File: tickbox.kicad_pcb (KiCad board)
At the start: 2 copper layers, 1 part, among them IC1 R5F10RLAGFB#10

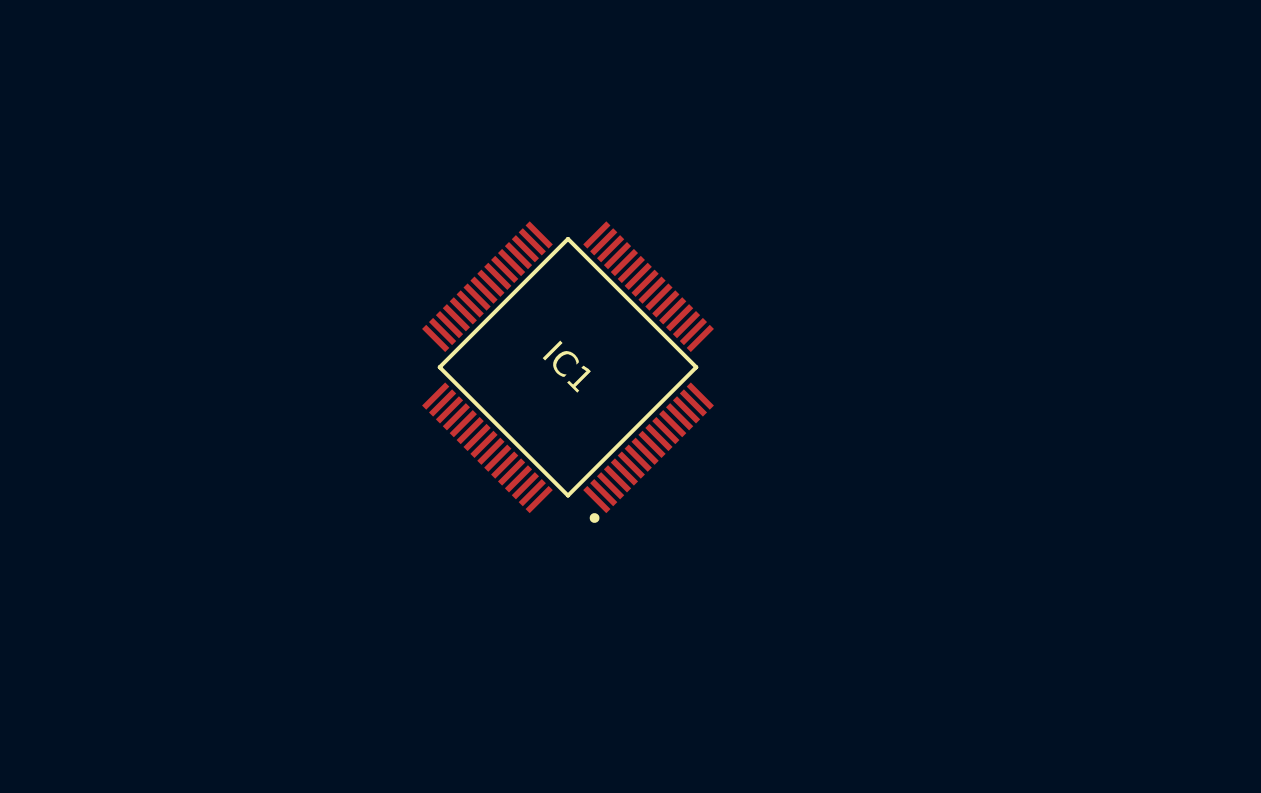
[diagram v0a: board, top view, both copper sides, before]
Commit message: Sketch PCB layout
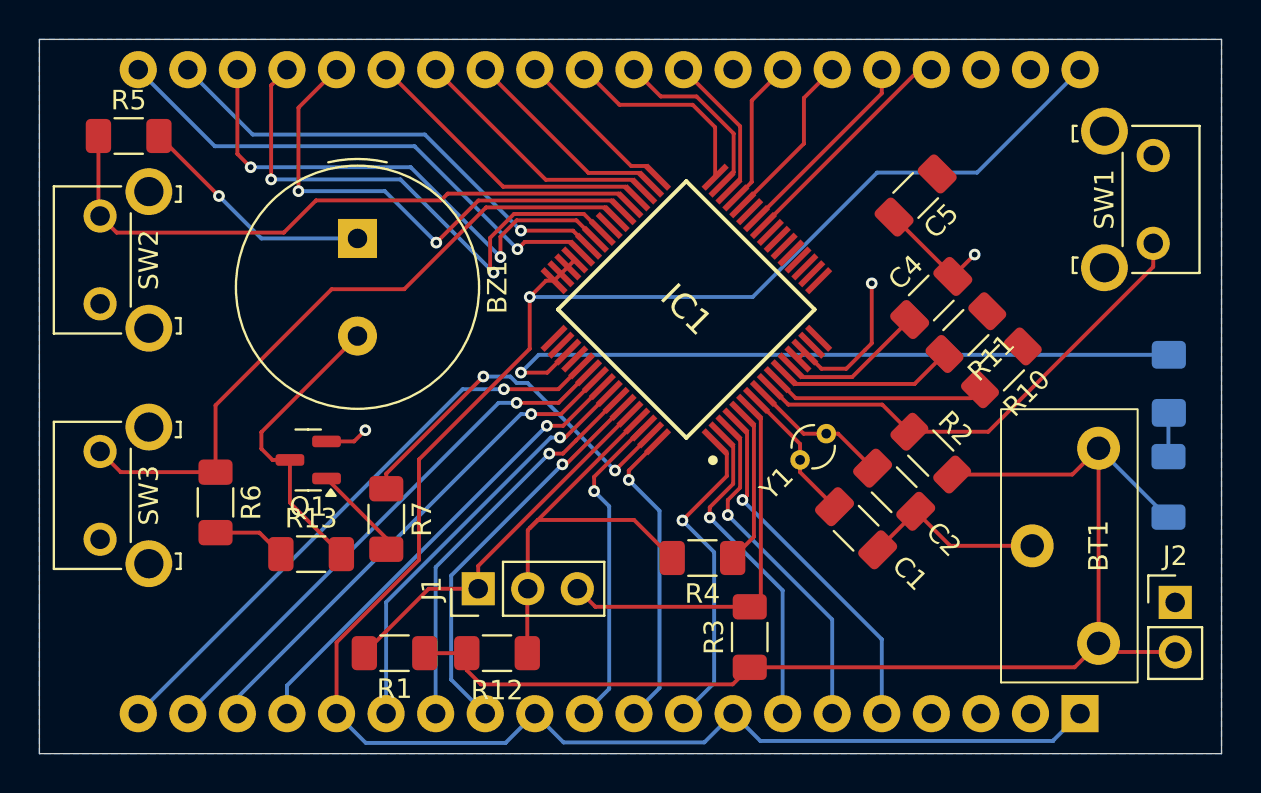
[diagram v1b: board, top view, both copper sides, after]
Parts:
- added BT1: Battery_Cell, 3rdparty:COIN_HOLDER_TH, F.Cu at (170.3, 109.9)
- added BZ1: Buzzer, Buzzer_Beeper:Buzzer_TDK_PS1240P02BT_D12.2mm_H6.5mm, F.Cu at (132.4, 94.2)
- added C1: 8pf, Capacitor_SMD:C_1206_3216Metric_Pad1.33x1.80mm_HandSolder, F.Cu at (157.9, 109.0)
- added C2: 8pf, Capacitor_SMD:C_1206_3216Metric_Pad1.33x1.80mm_HandSolder, F.Cu at (159.9, 107.0)
- added C4: 0.47uF, Capacitor_SMD:C_1206_3216Metric_Pad1.33x1.80mm_HandSolder, F.Cu at (161.8, 97.2)
- added C5: 0.1uF, Capacitor_SMD:C_1206_3216Metric_Pad1.33x1.80mm_HandSolder, F.Cu at (161.0, 92.0)
- added D1: ~, 3rdparty:VI-402, B.Cu at (144.0, 87.5)
- added D2: LED, LED_SMD:LED_1206_3216Metric_Pad1.42x1.75mm_HandSolder, B.Cu at (173.9, 101.6)
- added J1: Conn_01x03_Pin, Connector_PinHeader_2.54mm:PinHeader_1x03_P2.54mm_Vertical, F.Cu at (138.6, 112.1)
- added J2: Conn_01x02_Pin, Connector_PinHeader_2.54mm:PinHeader_1x02_P2.54mm_Vertical, F.Cu at (174.3, 112.8)
- added Q1: BC848, Package_TO_SOT_SMD:SOT-23, F.Cu at (129.8, 105.5)
- added R1: 10k, Resistor_SMD:R_1206_3216Metric_Pad1.30x1.75mm_HandSolder, F.Cu at (134.3, 115.4)
- added R10: 10k, Resistor_SMD:R_1206_3216Metric_Pad1.30x1.75mm_HandSolder, F.Cu at (165.4, 100.8)
- added R11: 10k, Resistor_SMD:R_1206_3216Metric_Pad1.30x1.75mm_HandSolder, F.Cu at (163.6, 99.0)
- added R12: 10k, Resistor_SMD:R_1206_3216Metric_Pad1.30x1.75mm_HandSolder, F.Cu at (139.5, 115.4)
- added R13: 1k, Resistor_SMD:R_1206_3216Metric_Pad1.30x1.75mm_HandSolder, F.Cu at (130.0, 110.3)
- added R2: 10k, Resistor_SMD:R_1206_3216Metric_Pad1.30x1.75mm_HandSolder, F.Cu at (161.8, 105.2)
- added R3: 1k, Resistor_SMD:R_1206_3216Metric_Pad1.30x1.75mm_HandSolder, F.Cu at (152.5, 114.6)
- added R4: 2k, Resistor_SMD:R_1206_3216Metric_Pad1.30x1.75mm_HandSolder, F.Cu at (150.1, 110.5)
- added R5: 10k, Resistor_SMD:R_1206_3216Metric_Pad1.30x1.75mm_HandSolder, F.Cu at (120.7, 88.9)
- added R6: 10k, Resistor_SMD:R_1206_3216Metric_Pad1.30x1.75mm_HandSolder, F.Cu at (125.1, 107.7)
- added R7: 4.7k, Resistor_SMD:R_1206_3216Metric_Pad1.30x1.75mm_HandSolder, F.Cu at (133.8, 108.5)
- added R9: 1.6k, Resistor_SMD:R_1206_3216Metric_Pad1.30x1.75mm_HandSolder, B.Cu at (173.9, 106.9)
- added SW1: SW_MEC_5G, Button_Switch_THT:SW_SPST_Omron_B3F-315x_Angled, F.Cu at (173.2, 89.9)
- added SW2: SW_MEC_5G, Button_Switch_THT:SW_SPST_Omron_B3F-315x_Angled, F.Cu at (119.2, 97.5)
- added SW3: SW_MEC_5G, Button_Switch_THT:SW_SPST_Omron_B3F-315x_Angled, F.Cu at (119.2, 109.6)
- added Y1: 32.768 kHz, Crystal:Crystal_DS26_D2.0mm_L6.0mm_Vertical, F.Cu at (156.4, 104.2)
- moved IC1 6.75 mm to (149.2, 97.8)
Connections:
- IC1 pad 10: unconnected-(IC1-P122/X2/EXCLK-Pad10) -> Net-(IC1-P122/X2/EXCLK)
- IC1 pad 11: unconnected-(IC1-P121/X1-Pad11) -> Net-(IC1-P121/X1)
- IC1 pad 19: unconnected-(IC1-P127/CAPH-Pad19) -> /SWIN
- IC1 pad 20: unconnected-(IC1-P126/CAPL-Pad20) -> /SWOUT
- IC1 pad 37: unconnected-(IC1-P50/INTP5/SEG7/(PCLBUZ0)-Pad37) -> Net-(IC1-P50/INTP5/SEG7/(PCLBUZ0))
- IC1 pad 39: unconnected-(IC1-P16/SI01/INTP2/SEG5-Pad39) -> Net-(IC1-P16/SI01/INTP2/SEG5)
- IC1 pad 51: unconnected-(IC1-P130-Pad51) -> Net-(D2-K)
- IC1 pad 63: unconnected-(IC1-P140/TO00/PCLBUZ0/SEG27/(INTP6)-Pad63) -> /PCLBUZ0
- IC1 pad 9: unconnected-(IC1-P137/INTP0-Pad9) -> Net-(IC1-P137/INTP0)
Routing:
- net /COM: track 0.00 -> 103.3 mm, vias 0 -> 1
- net VDD: track 0.00 -> 80.3 mm, vias 0 -> 1
- net Net-(D2-K): track 0.00 -> 36.4 mm, vias 0 -> 1
- net Net-(IC1-P16/SI01/INTP2/SEG5): track 0.00 -> 34.7 mm
- net Net-(IC1-P50/INTP5/SEG7/(PCLBUZ0)): track 0.00 -> 32.7 mm
- net /SEG37: track 0.00 -> 30.1 mm, vias 0 -> 1
- net /SEG3: track 0.00 -> 27.9 mm, vias 0 -> 2
- net /SEG36: track 0.00 -> 27.8 mm, vias 0 -> 1
- net /SEG0: track 0.00 -> 26.9 mm, vias 0 -> 1
- net /SEG2: track 0.00 -> 26.6 mm, vias 0 -> 2
- net /SEG6: track 0.00 -> 26.0 mm, vias 0 -> 2
- net /SEG35: track 0.00 -> 25.9 mm, vias 0 -> 1
- net GND: track 0.00 -> 25.5 mm, vias 0 -> 3
- net Net-(IC1-P137/INTP0): track 0.00 -> 25.3 mm
- net /SEG1: track 0.00 -> 24.3 mm, vias 0 -> 1
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- added copper zone on B.Cu, net GND
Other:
- board outline added: 60.6 x 36.6 mm
- copper layers 2 -> 4
